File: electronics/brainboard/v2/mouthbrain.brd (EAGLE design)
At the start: 76.8 x 53.3 mm, 29 parts, among them Q1 MOSFET-NCHANNELSMD, Q10 MOSFET-NCHANNELSMD, Q11 MOSFET-NCHANNELSMD, Q12 MOSFET-NCHANNELSMD, Q13 MOSFET-NCHANNELSMD, Q14 MOSFET-NCHANNELSMD, Q15 MOSFET-NCHANNELSMD, Q16 MOSFET-NCHANNELSMD, Q2 MOSFET-NCHANNELSMD, Q3 MOSFET-NCHANNELSMD, Q4 MOSFET-NCHANNELSMD, Q5 MOSFET-NCHANNELSMD, Q6 MOSFET-NCHANNELSMD, Q7 MOSFET-NCHANNELSMD, Q8 MOSFET-NCHANNELSMD, Q9 MOSFET-NCHANNELSMD, U1 MCP4352, U2 MCP4352, U3 MCP4352, U4 MCP4352, U5 MOSFET-NCHANNEL-SOIC8

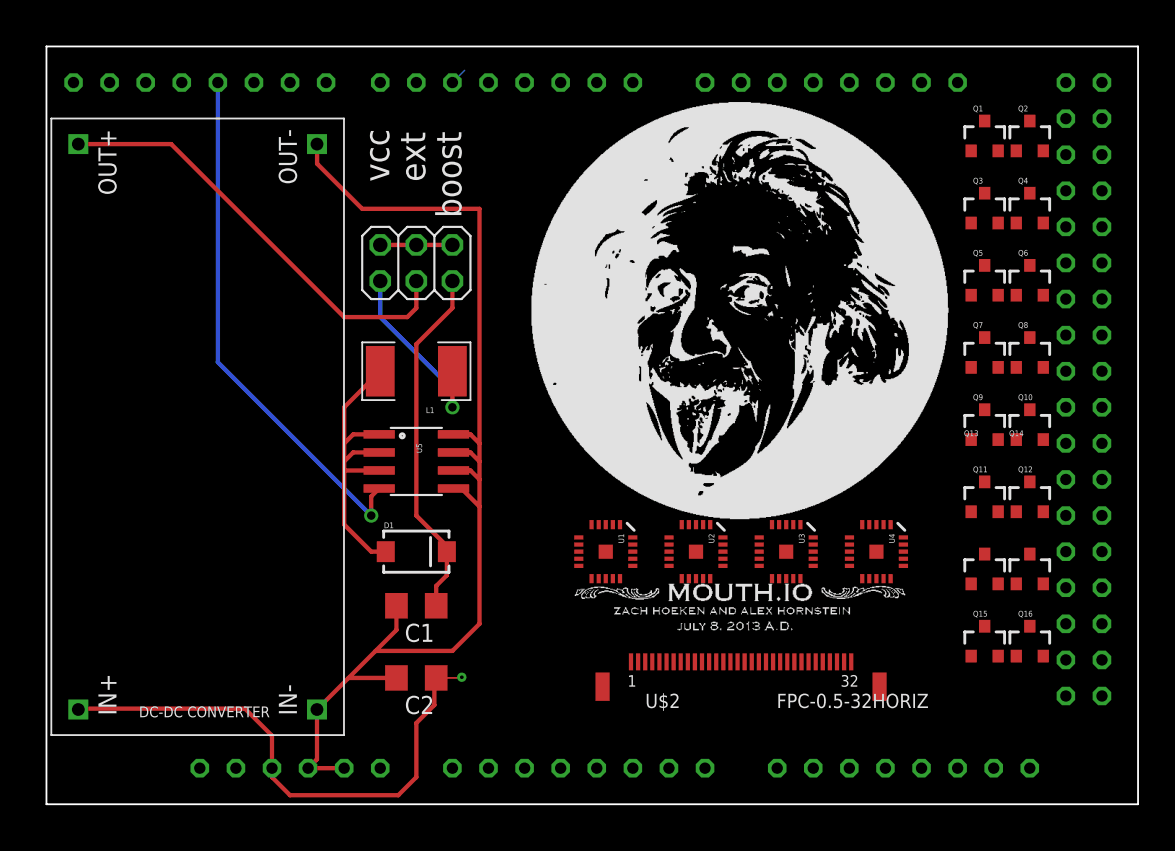
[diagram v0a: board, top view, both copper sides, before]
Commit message: mouthbrain ready for prototyping.
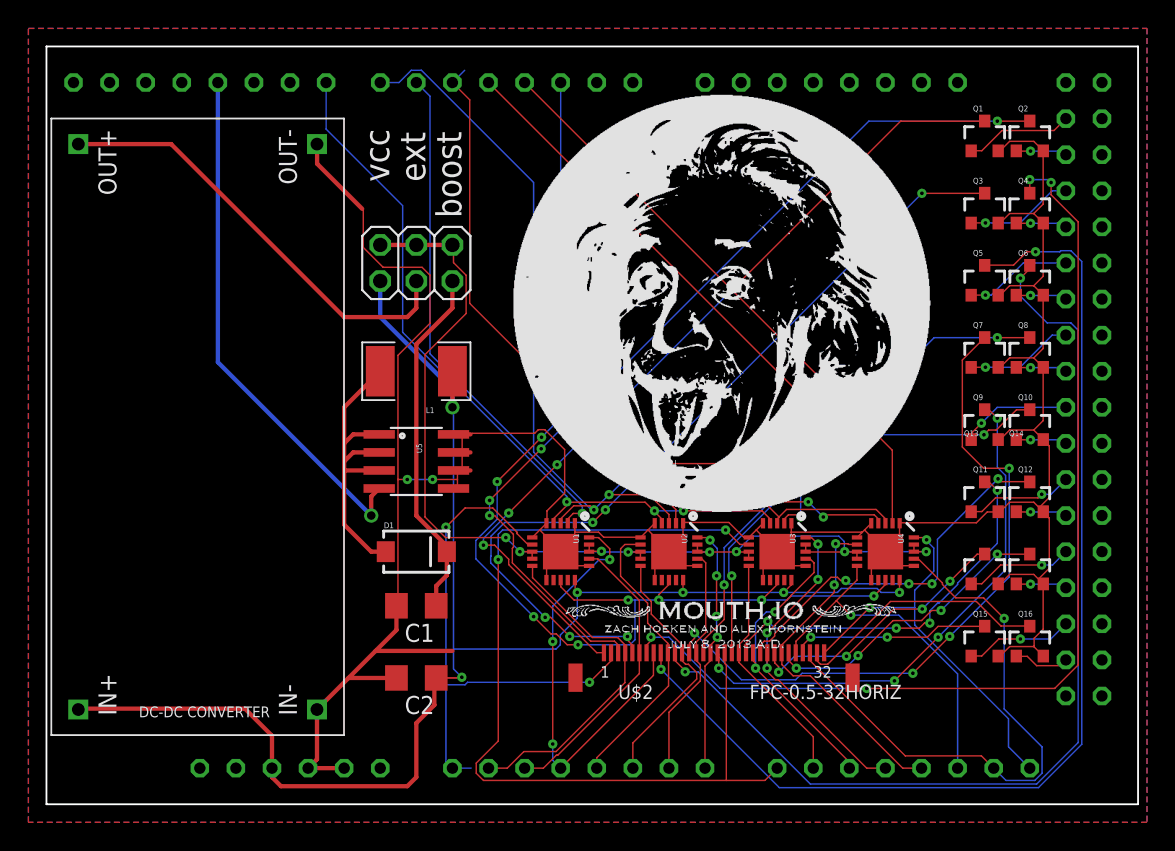
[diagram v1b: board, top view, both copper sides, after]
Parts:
- moved U1 3.17 mm to (36.2, 17.8)
- moved U$2 2.01 mm to (47.0, 10.2)
- moved U2 1.91 mm to (43.8, 17.8)
- moved U3 0.63 mm to (51.4, 17.8)
- moved U4 0.63 mm to (59.1, 17.8)
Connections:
- net GND: now also U1.0, U2.0, U3.0, U4.0
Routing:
- net GND: track 80.0 -> 221.0 mm, vias 0 -> 2
- net !RESET: track 0.00 -> 80.7 mm, vias 0 -> 8
- net COUT4: track 0.00 -> 77.1 mm, vias 0 -> 2
- net SCK: track 0.00 -> 72.6 mm, vias 0 -> 3
- net VDD: track 5.08 -> 76.5 mm, vias 0 -> 8
- net COUT3: track 0.00 -> 70.8 mm, vias 0 -> 4
- net COUT5: track 0.00 -> 70.3 mm, vias 0 -> 2
- net SI: track 0.00 -> 70.0 mm, vias 0 -> 6
- net AOUT8: track 0.00 -> 66.4 mm, vias 0 -> 2
- net COUT1: track 0.00 -> 64.8 mm, vias 0 -> 4
- net COUT0: track 0.00 -> 59.8 mm, vias 0 -> 4
- net COUT2: track 0.00 -> 59.7 mm, vias 0 -> 6
- net VCC: track 51.5 -> 108.8 mm, vias 2 -> 6
- net COUT6: track 0.00 -> 48.0 mm, vias 0 -> 4
- net !CS4: track 0.00 -> 41.8 mm
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- added copper zone on layer 1, net GND
- added copper zone on layer 16, net GND
